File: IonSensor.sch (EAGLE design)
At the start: 20 parts, among them IC1 QUAD_OPAMPD, IC2 QUAD_OPAMPD, IC3 QUAD_OPAMPD, X1 JST-XH-04-PIN-LONG-PAD

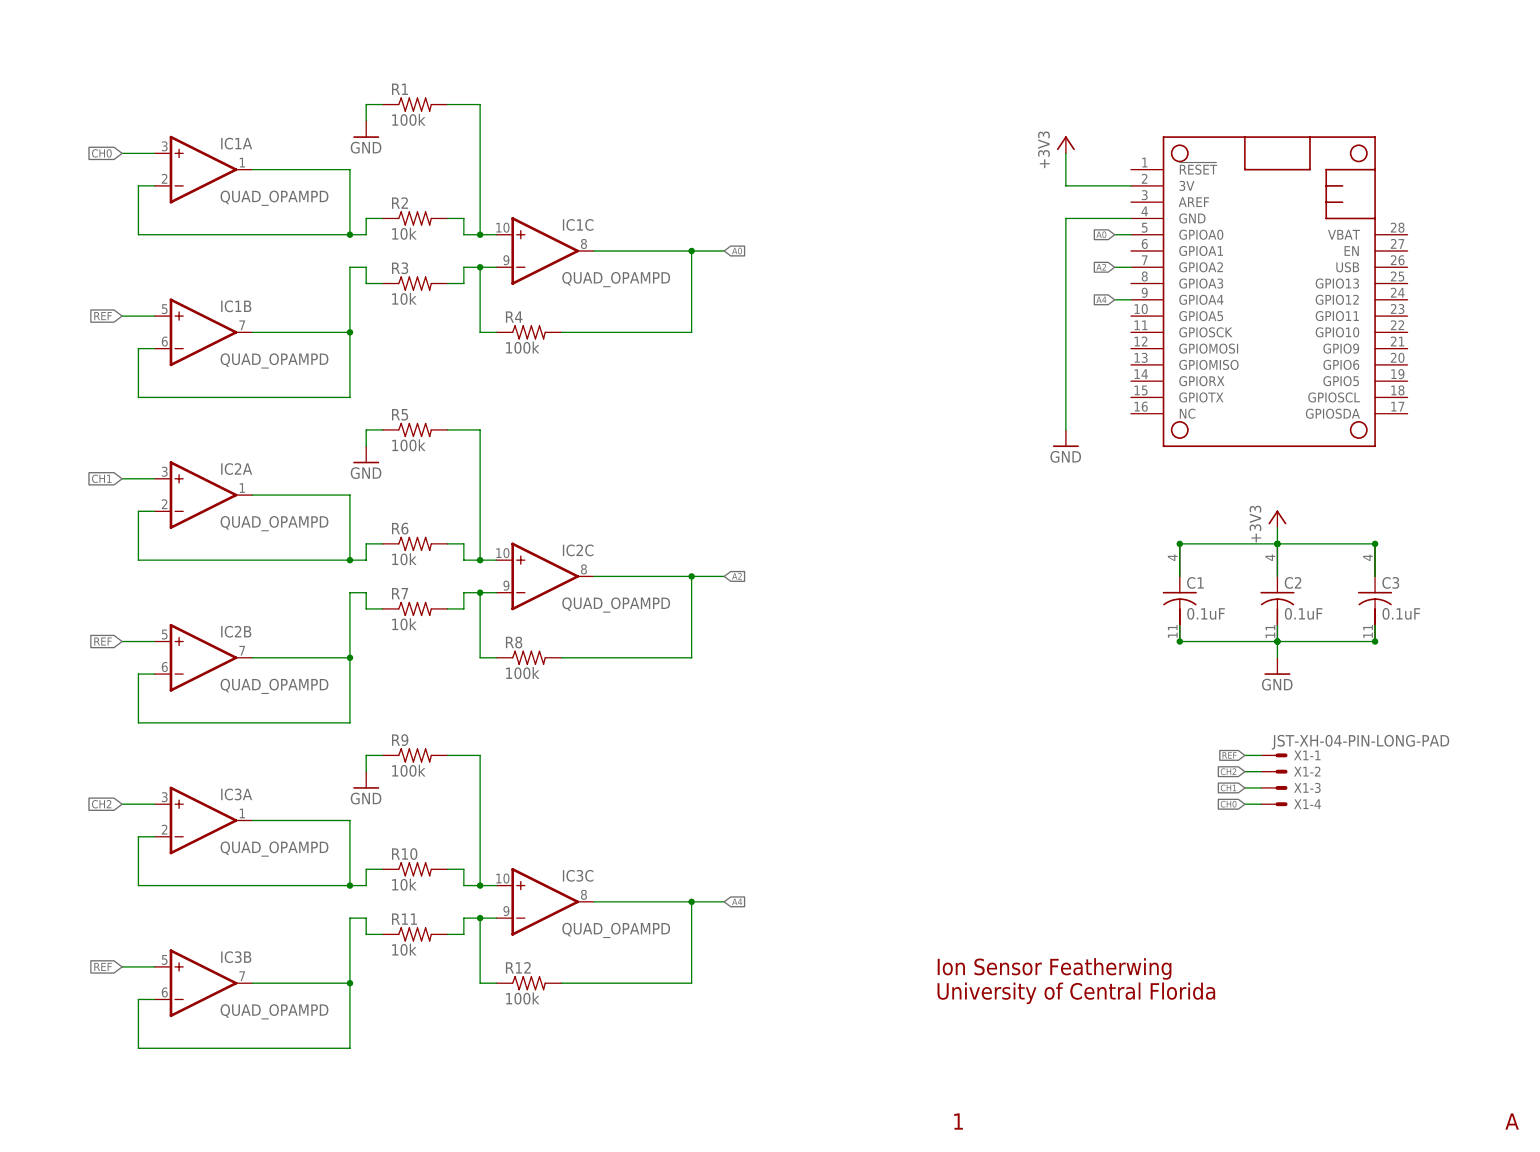
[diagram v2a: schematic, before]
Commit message: Rev. D
Upgrade to Rev. D, no connector
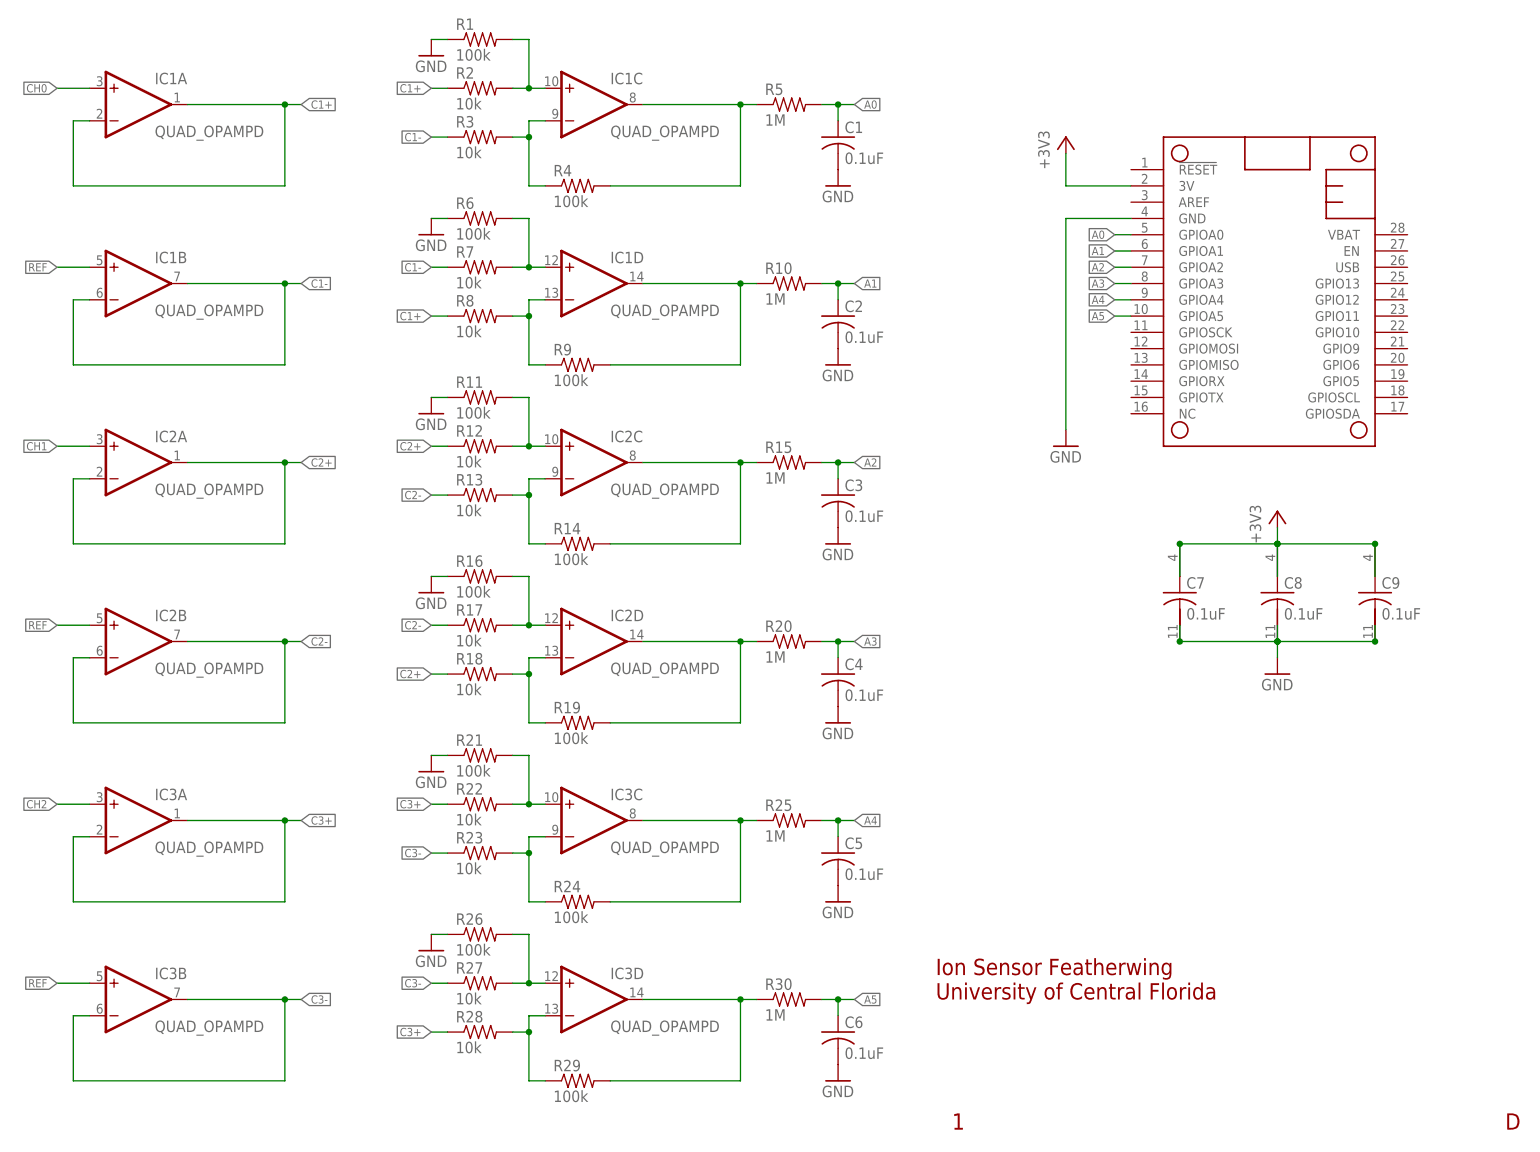
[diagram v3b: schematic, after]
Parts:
- removed X1: JST-XH-04-PIN-LONG-PAD, Rembrandt Electronics - JST XH Connectors v1-0:JST-XH-04-PIN-LONG-PAD
- added C4, C5, C6, C7, C8, C9: 0.1uF, adafruit:C-USC0402
- added R13, R17, R18, R22, R23, R27, R28: 10k, adafruit:R-US_R0402
- added R14, R16, R19, R21, R24, R26, R29: 100k, adafruit:R-US_R0402
- added R15, R20, R25, R30: 1M, adafruit:R-US_R0402
- C1, C2, C3: device adafruit:C-USC0603 -> adafruit:C-USC0402
- R1, R2, R3, R4, R7, R9: device adafruit:R-US_R0603 -> adafruit:R-US_R0402
- R10: value 10k -> 1M; device adafruit:R-US_R0603 -> adafruit:R-US_R0402
- R11, R6: value 10k -> 100k; device adafruit:R-US_R0603 -> adafruit:R-US_R0402
- R12, R8: value 100k -> 10k; device adafruit:R-US_R0603 -> adafruit:R-US_R0402
- R5: value 100k -> 1M; device adafruit:R-US_R0603 -> adafruit:R-US_R0402
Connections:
- removed net N$1 (its old number): IC1A.-IN, IC1A.OUT, R2.1
- new net A1: C2.1, MS1.GPIOA1, R10.2
- new net A3: C4.1, MS1.GPIOA3, R20.2
- new net A5: C6.1, MS1.GPIOA5, R30.2
- new net C1+: IC1A.-IN, IC1A.OUT, R2.1, R8.1
- new net C1-: IC1B.-IN, IC1B.OUT, R3.1, R7.1
- new net C2+: IC2A.-IN, IC2A.OUT, R12.1, R18.1
- new net C2-: IC2B.-IN, IC2B.OUT, R13.1, R17.1
- new net C3+: IC3A.-IN, IC3A.OUT, R22.1, R28.1
- new net C3-: IC3B.-IN, IC3B.OUT, R23.1, R27.1
- new net N$10: IC1D.OUT, R10.1, R9.2
- new net N$15: IC3D.-IN, R28.2, R29.1
- new net N$16: IC2D.OUT, R19.2, R20.1
- new net N$17: IC3C.OUT, R24.2, R25.1
- new net N$18: IC3D.OUT, R29.2, R30.1
- new net N$4: IC1D.+IN, R6.2, R7.2
- new net N$5: IC1C.OUT, R4.2, R5.1
- net +3V3: now also C7.1, C8.1, C9.1; no longer C1.1, C2.1, C3.1
- net A0: now also C1.1, R5.2; no longer IC1C.OUT, R4.2
- net A2: now also C3.1, R15.2; no longer IC2C.OUT, R8.2
- net A4: now also C5.1, R25.2; no longer IC3C.OUT, R12.2
- net CH0: no longer X1-4.S
- net CH1: no longer X1-3.S
- net CH2: no longer X1-2.S
- net GND: now also C4.2, C5.2, C6.2, C7.2, C8.2, C9.2, R11.1, R16.1, R21.1, R26.1, R6.1; no longer R5.1, R9.1
- net N$11: now also IC2D.+IN, R16.2, R17.2; no longer IC3A.-IN, IC3A.OUT, R10.1
- net N$12: now also IC3D.+IN, R26.2, R27.2; no longer IC3B.-IN, IC3B.OUT, R11.1
- net N$13: now also IC2D.-IN, R18.2, R19.1; no longer IC3C.+IN, R10.2, R9.2
- net N$14: now also IC2C.OUT, R14.2, R15.1; no longer IC3C.-IN, R11.2, R12.1
- net N$3: now also IC3C.+IN, R21.2, R22.2; no longer IC1B.-IN, IC1B.OUT, R3.1
- net N$6: now also IC1D.-IN, R8.2, R9.1; no longer IC2A.-IN, IC2A.OUT, R6.1
- net N$7: now also IC3C.-IN, R23.2, R24.1; no longer IC2B.-IN, IC2B.OUT, R7.1
- net N$8: now also R11.2, R12.2; no longer R5.2, R6.2
- net N$9: now also R13.2, R14.1; no longer R7.2, R8.1
- net REF: no longer X1-1.S
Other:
- note added: "D"
- note removed: "A"
- moved on the sheet: C1, C2, C3, IC1A, IC1B, IC1C, IC2A, IC2B, IC2C, IC3A, IC3B, IC3C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

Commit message: Revert "Rev. D"
This reverts commit b0cd00c38bcd6b0f7db002c888a5e278bdb202ce.
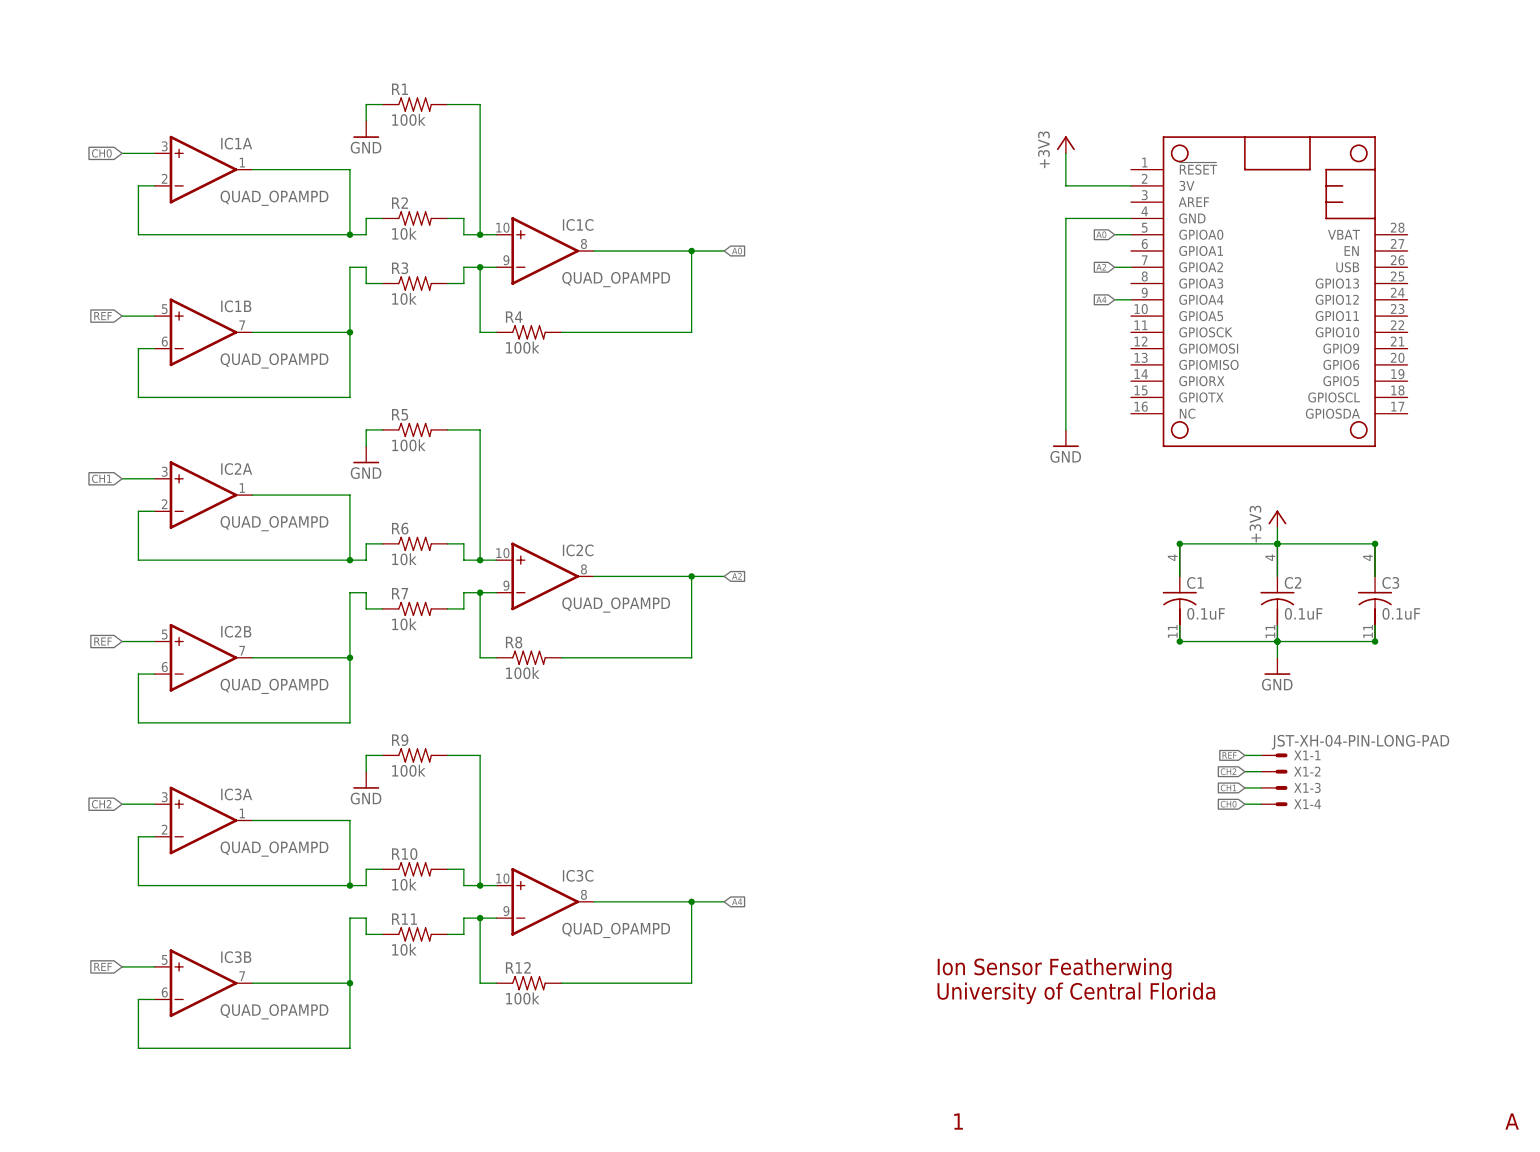
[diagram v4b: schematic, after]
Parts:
- removed C4, C5, C6, C7, C8, C9: 0.1uF, adafruit:C-USC0402
- removed R13, R17, R18, R22, R23, R27, R28: 10k, adafruit:R-US_R0402
- removed R14, R16, R19, R21, R24, R26, R29: 100k, adafruit:R-US_R0402
- removed R15, R20, R25, R30: 1M, adafruit:R-US_R0402
- added X1: JST-XH-04-PIN-LONG-PAD, Rembrandt Electronics - JST XH Connectors v1-0:JST-XH-04-PIN-LONG-PAD
- C1, C2, C3: device adafruit:C-USC0402 -> adafruit:C-USC0603
- R1, R2, R3, R4, R7, R9: device adafruit:R-US_R0402 -> adafruit:R-US_R0603
- R10: value 1M -> 10k; device adafruit:R-US_R0402 -> adafruit:R-US_R0603
- R11, R6: value 100k -> 10k; device adafruit:R-US_R0402 -> adafruit:R-US_R0603
- R12, R8: value 10k -> 100k; device adafruit:R-US_R0402 -> adafruit:R-US_R0603
- R5: value 1M -> 100k; device adafruit:R-US_R0402 -> adafruit:R-US_R0603
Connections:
- removed net A1: C2.1, MS1.GPIOA1, R10.2
- removed net A3: C4.1, MS1.GPIOA3, R20.2
- removed net A5: C6.1, MS1.GPIOA5, R30.2
- removed net C1+: IC1A.-IN, IC1A.OUT, R2.1, R8.1
- removed net C1-: IC1B.-IN, IC1B.OUT, R3.1, R7.1
- removed net C2+: IC2A.-IN, IC2A.OUT, R12.1, R18.1
- removed net C2-: IC2B.-IN, IC2B.OUT, R13.1, R17.1
- removed net C3+: IC3A.-IN, IC3A.OUT, R22.1, R28.1
- removed net C3-: IC3B.-IN, IC3B.OUT, R23.1, R27.1
- removed net N$10: IC1D.OUT, R10.1, R9.2
- removed net N$15: IC3D.-IN, R28.2, R29.1
- removed net N$16: IC2D.OUT, R19.2, R20.1
- removed net N$17: IC3C.OUT, R24.2, R25.1
- removed net N$18: IC3D.OUT, R29.2, R30.1
- removed net N$4 (its old number): IC1D.+IN, R6.2, R7.2
- removed net N$5: IC1C.OUT, R4.2, R5.1
- new net N$1: IC1A.-IN, IC1A.OUT, R2.1
- net +3V3: now also C1.1, C2.1, C3.1; no longer C7.1, C8.1, C9.1
- net A0: now also IC1C.OUT, R4.2; no longer C1.1, R5.2
- net A2: now also IC2C.OUT, R8.2; no longer C3.1, R15.2
- net A4: now also IC3C.OUT, R12.2; no longer C5.1, R25.2
- net CH0: now also X1-4.S
- net CH1: now also X1-3.S
- net CH2: now also X1-2.S
- net GND: now also R5.1, R9.1; no longer C4.2, C5.2, C6.2, C7.2, C8.2, C9.2, R11.1, R16.1, R21.1, R26.1, R6.1
- net N$11: now also IC3A.-IN, IC3A.OUT, R10.1; no longer IC2D.+IN, R16.2, R17.2
- net N$12: now also IC3B.-IN, IC3B.OUT, R11.1; no longer IC3D.+IN, R26.2, R27.2
- net N$13: now also IC3C.+IN, R10.2, R9.2; no longer IC2D.-IN, R18.2, R19.1
- net N$14: now also IC3C.-IN, R11.2, R12.1; no longer IC2C.OUT, R14.2, R15.1
- net N$3: now also IC1B.-IN, IC1B.OUT, R3.1; no longer IC3C.+IN, R21.2, R22.2
- net N$6: now also IC2A.-IN, IC2A.OUT, R6.1; no longer IC1D.-IN, R8.2, R9.1
- net N$7: now also IC2B.-IN, IC2B.OUT, R7.1; no longer IC3C.-IN, R23.2, R24.1
- net N$8: now also R5.2, R6.2; no longer R11.2, R12.2
- net N$9: now also R7.2, R8.1; no longer R13.2, R14.1
- net REF: now also X1-1.S
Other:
- note added: "A"
- note removed: "D"
- moved on the sheet: C1, C2, C3, IC1A, IC1B, IC1C, IC2A, IC2B, IC2C, IC3A, IC3B, IC3C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
